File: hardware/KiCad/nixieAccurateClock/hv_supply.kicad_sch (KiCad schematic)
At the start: 3 parts, among them J10 Conn_01x02_Pin

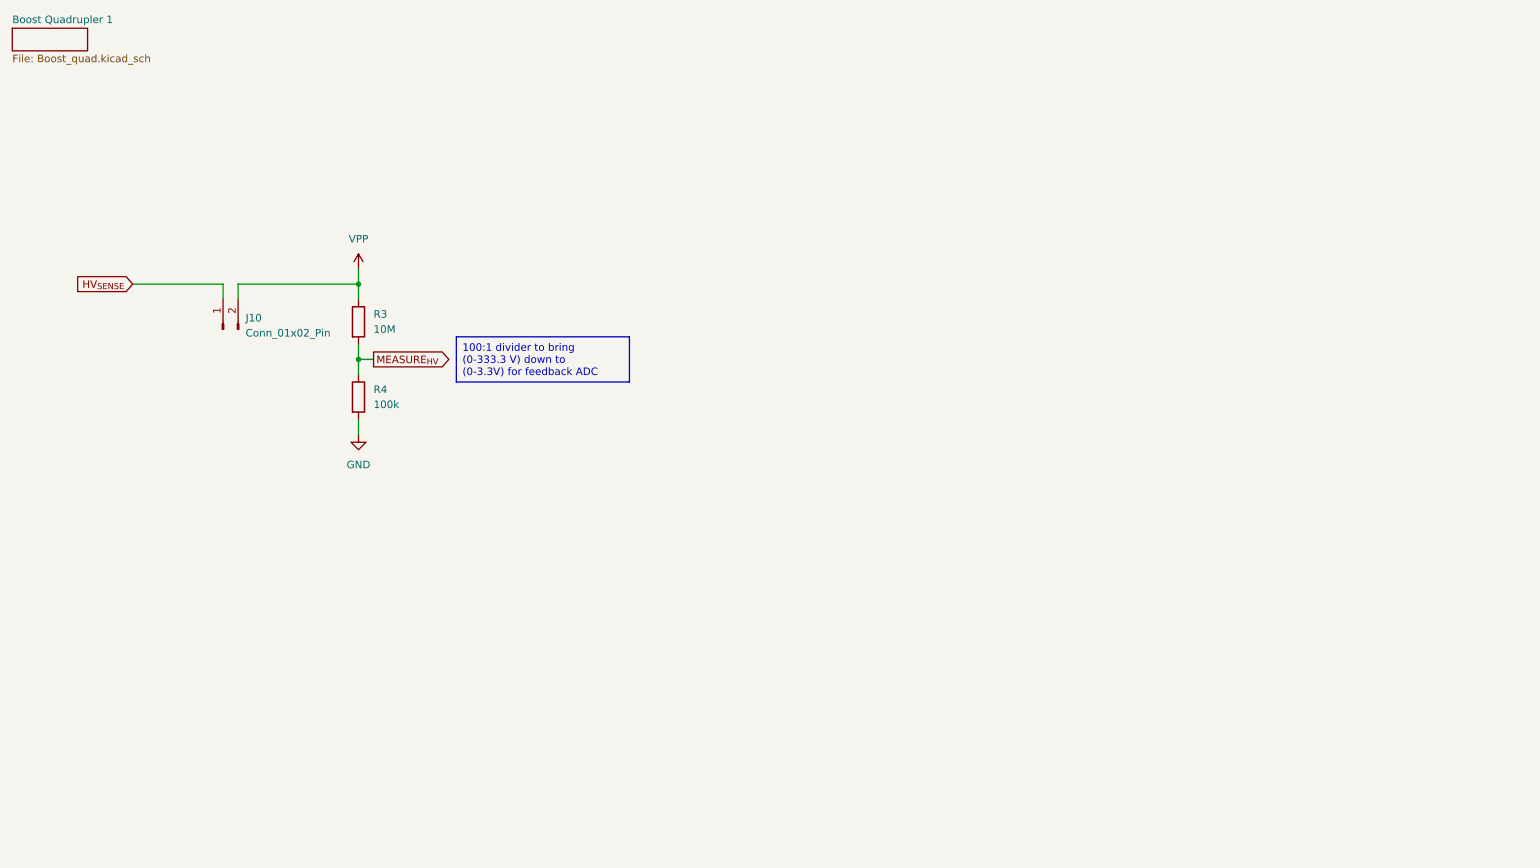
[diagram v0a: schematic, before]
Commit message: proper HVPS
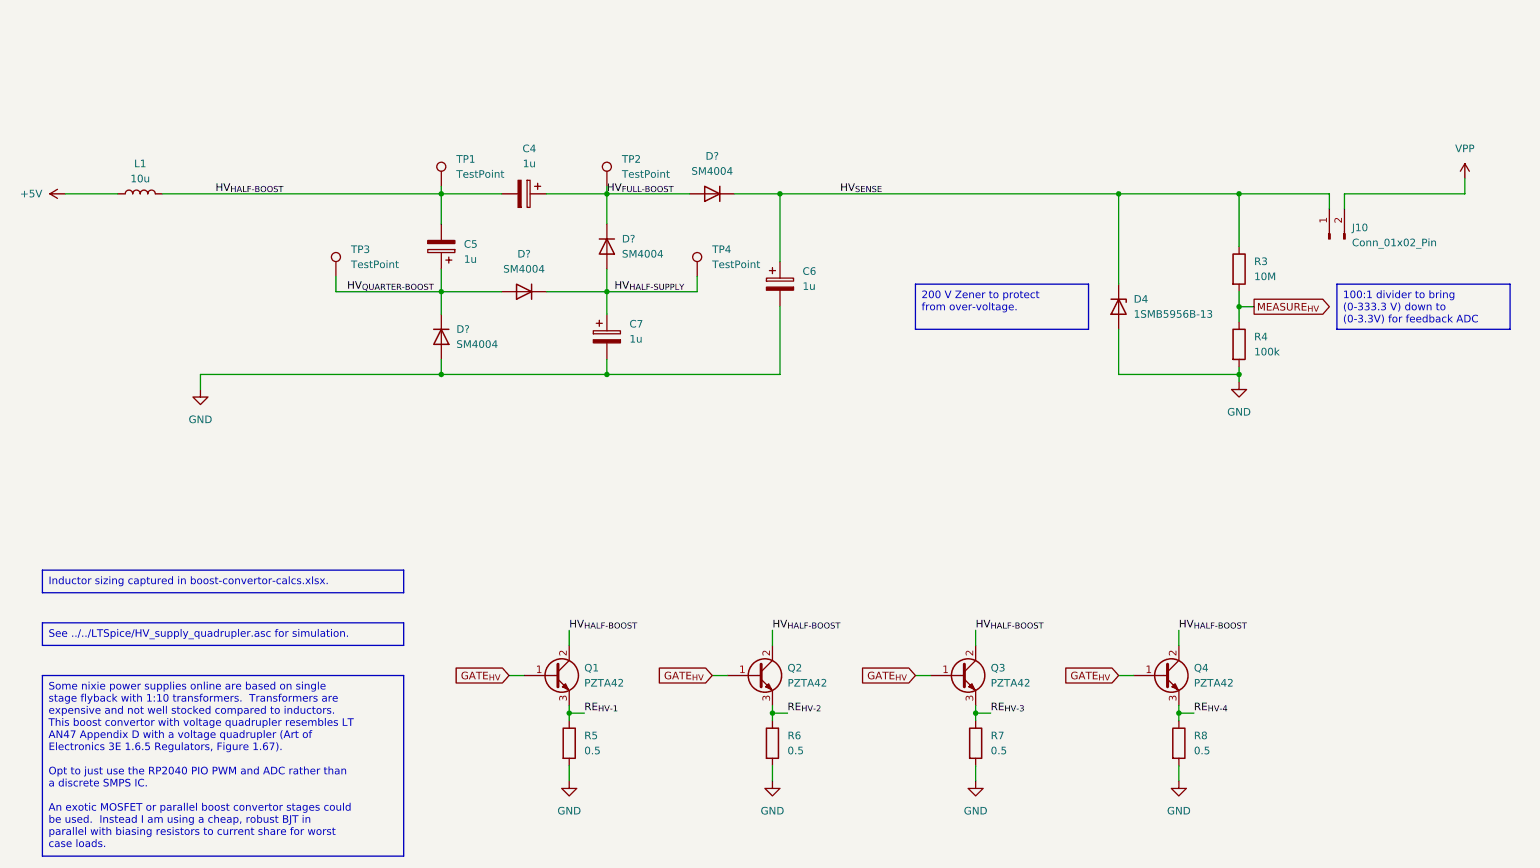
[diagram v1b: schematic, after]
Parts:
- added C4, C5, C6, C7: 1u, Capacitor_SMD:CP_Elec_8x10, symbol Device:C_Polarized
- added D4: 1SMB5956B-13, Diode_SMD:D_SMB, symbol Device:D_Zener
- added D? (x4): SM4004, Diode_SMD:D_MELF, symbol Diode:SM4004
- added L1: 10u, 00_lib:IND_BOURNS_SRR1280, symbol Device:L
- added Q1, Q2, Q3, Q4: PZTA42, Package_TO_SOT_SMD:SOT-223-3_TabPin2, symbol Transistor_BJT:PZTA42
- added R5, R6, R7, R8: 0.5, Resistor_SMD:R_2010_5025Metric, symbol Device:R
- added TP1, TP2, TP3, TP4: TestPoint, 00_lib:TestPoint_Keystone_5019_Minature, symbol Connector:TestPoint
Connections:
- net GND: now also C6.2, C7.2, D4.2 (A), D?.2 (A), R5.2, R6.2, R7.2, R8.2
- net HV_{SENSE}: now also R3.1, C6.1, D4.1 (K), D?.1 (K)
- net VPP: no longer R3.1
- new net +5V: L1.1
- new net GATE_{HV}: Q1.1 (B), Q2.1 (B), Q3.1 (B), Q4.1 (B)
- new net HV_{FULL-BOOST}: C4.1, D?.1 (K), D?.2 (A), TP2.1
- new net HV_{HALF-BOOST}: C4.2, C5.2, L1.2, Q1.2 (C), Q2.2 (C), Q3.2 (C), Q4.2 (C), TP1.1
- new net HV_{HALF-SUPPLY}: C7.1, D?.1 (K), D?.2 (A), TP4.1
- new net HV_{QUARTER-BOOST}: C5.1, D?.1 (K), D?.2 (A), TP3.1
- new net RE_{HV-1}: Q1.3 (E), R5.1
- new net RE_{HV-2}: Q2.3 (E), R6.1
- new net RE_{HV-3}: Q3.3 (E), R7.1
- new net RE_{HV-4}: Q4.3 (E), R8.1
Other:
- removed sheet Boost Quadrupler 1
- moved on the sheet: J10, R3, R4
